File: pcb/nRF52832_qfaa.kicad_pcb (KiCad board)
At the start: 4 copper layers, 40 x 20 mm, 118 parts, among them J1 Conn_01x01_Female, J3 USB_B_Micro, J4 Conn_01x02_Socket, J5 Conn_01x03_Socket, U2 W25Q32JVZP, U3 TPS63802DLAR, U4 BQ24078RGTR, U5 RV-4162-C7, U6 SN74LVC1G79DBVT, U7 NRF5340-QKAA-R7, X1 32.768kHz, X2 32MHz

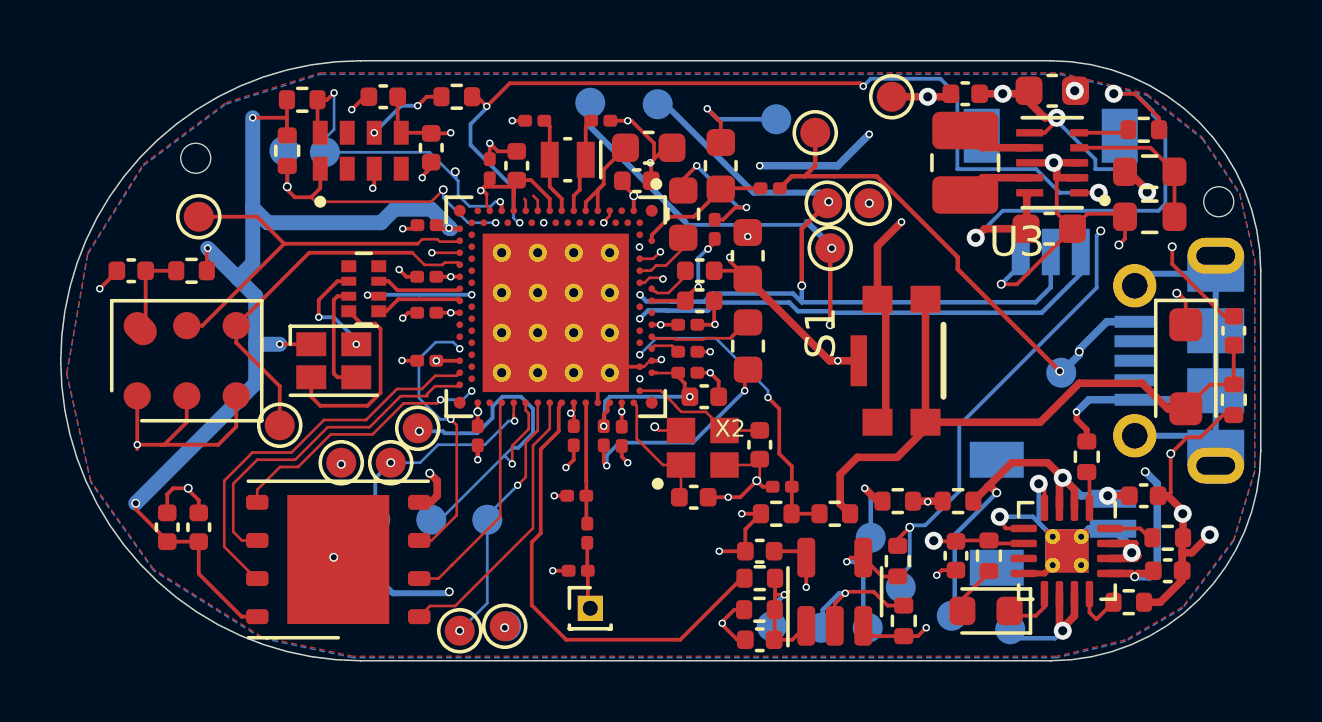
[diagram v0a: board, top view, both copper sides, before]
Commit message: finalizing 1.4, going for the dry run
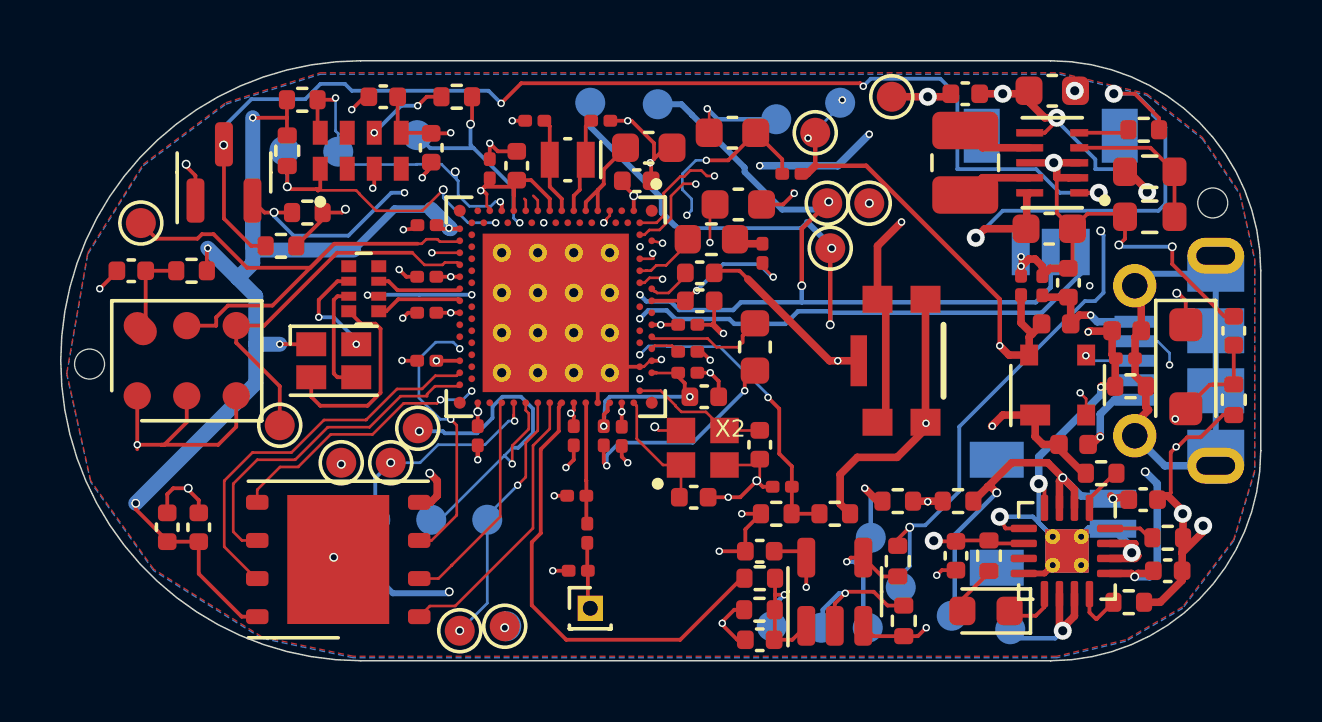
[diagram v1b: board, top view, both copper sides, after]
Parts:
- added C5: 100n, Capacitor_SMD:C_0201_0603Metric, F.Cu at (147.7, 96.5)
- added C6: 1u, Capacitor_SMD:C_0402_1005Metric, F.Cu at (148.6, 96.4)
- added C7: 100n, Capacitor_SMD:C_0201_0603Metric, F.Cu at (147.0, 96.5)
- added C8: 100n, Capacitor_SMD:C_0201_0603Metric, F.Cu at (150.5, 98.9)
- added D1: PRTR5V0U2X, Package_TO_SOT_SMD:SOT-143, F.Cu at (148.2, 99.8)
- added FB1: FerriteBead, Inductor_SMD:L_0402_1005Metric, F.Cu at (148.2, 97.8)
- added FB2: FerriteBead, Inductor_SMD:L_0402_1005Metric, F.Cu at (150.5, 98.0)
- added FB3: FerriteBead, Inductor_SMD:L_0402_1005Metric, F.Cu at (148.8, 101.8)
- added Q1: PMOS, Package_TO_SOT_SMD:SOT-23, F.Cu at (120.4, 92.7)
- added R22: 4.7k, Resistor_SMD:R_0402_1005Metric, F.Cu at (150.7, 99.8)
- added R23: 1M, Resistor_SMD:R_0402_1005Metric, F.Cu at (123.2, 94.1)
- added R24: 100K, Resistor_SMD:R_0402_1005Metric, F.Cu at (122.3, 95.2)
- added TP32: TestPoint, TestPoint:TestPoint_Pad_D1.0mm, B.Cu at (126.9, 91.5)
- U2: value W25Q32JVZP -> W25Q128JWPIQ
- moved TP2 11.6 mm to (141.0, 90.4)
- moved H2 7.72 mm to (116.0, 99.1)
- moved TP10 1.94 mm to (117.7, 94.4)
- moved L6 1.78 mm to (138.4, 95.4)
- moved C42 1.74 mm to (137.6, 93.8), turned to 0 degrees
- moved L4 1.26 mm to (136.7, 95.0), turned to 180 degrees
- moved C43 1.17 mm to (137.4, 91.4), turned to 180 degrees
- moved R20 0.87 mm to (139.4, 92.8)
- moved R7 0.73 mm to (149.7, 102.8), turned to 0 degrees
- moved TP5 0.45 mm to (124.2, 92.0)
- moved L3 0.23 mm to (138.1, 98.5)
- moved H1 0.20 mm to (153.4, 93.7)
- moved C20 0.13 mm to (151.1, 103.6)
- moved C44 0.07 mm to (136.3, 96.1)
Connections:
- J3 pad 1: V_charger -> Net-(J3-VBUS)
- J3 pad 2: unconnected-(J3-D--Pad2) -> /USB_N
- J3 pad 3: unconnected-(J3-D+-Pad3) -> /USB_P
- J3 pad 5: GND -> Net-(J3-GND)
- J3 pad 6: GND -> Net-(J3-Shield)
- R12 pad 1: VREG_EN -> /RTC_INT_N
- U7 pad AB2: VREG_EN -> /RTC_INT_N
- U7 pad B2: unconnected-(U7B-D+-PadB2) -> /USB_P
- U7 pad B4: unconnected-(U7B-D--PadB4) -> /USB_N
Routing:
- net /USB_N: track 0.00 -> 27.9 mm, vias 0 -> 3
- net /USB_P: track 0.00 -> 21.4 mm, vias 0 -> 2
- net Net-(J3-Shield): track 0.00 -> 18.3 mm
- net /RTC_INT_N: track 0.00 -> 17.9 mm, vias 0 -> 4
- net GND: track 254.5 -> 271.0 mm, vias 54 -> 59
- net VREG_EN: track 52.6 -> 61.9 mm
- net VSS: track 84.4 -> 91.5 mm, vias 7 -> 8
- net Net-(J3-VBUS): track 0.00 -> 4.16 mm, vias 0 -> 1
- net /PDM_DATA: track 13.6 -> 17.4 mm
- net Net-(U7A-VBUS): track 4.48 -> 8.08 mm, vias 0 -> 3
- net Net-(L4-Pad1): track 4.57 -> 1.03 mm, vias 2 -> 0
- net VCC: track 129.7 -> 132.8 mm
- net Net-(J3-GND): track 0.00 -> 2.75 mm, vias 0 -> 1
- net V_charger: track 28.4 -> 30.2 mm, vias 4 -> 5
- net Net-(U7A-DECD): track 3.45 -> 5.15 mm
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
